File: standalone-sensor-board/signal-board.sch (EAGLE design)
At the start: 32 parts, among them Q1 QRE1113, Q2 QRE1113, Q3 QRE1113, Q4 QRE1113, Q5 QRE1113, Q6 QRE1113, Q7 QRE1113, U1 CD4051BE

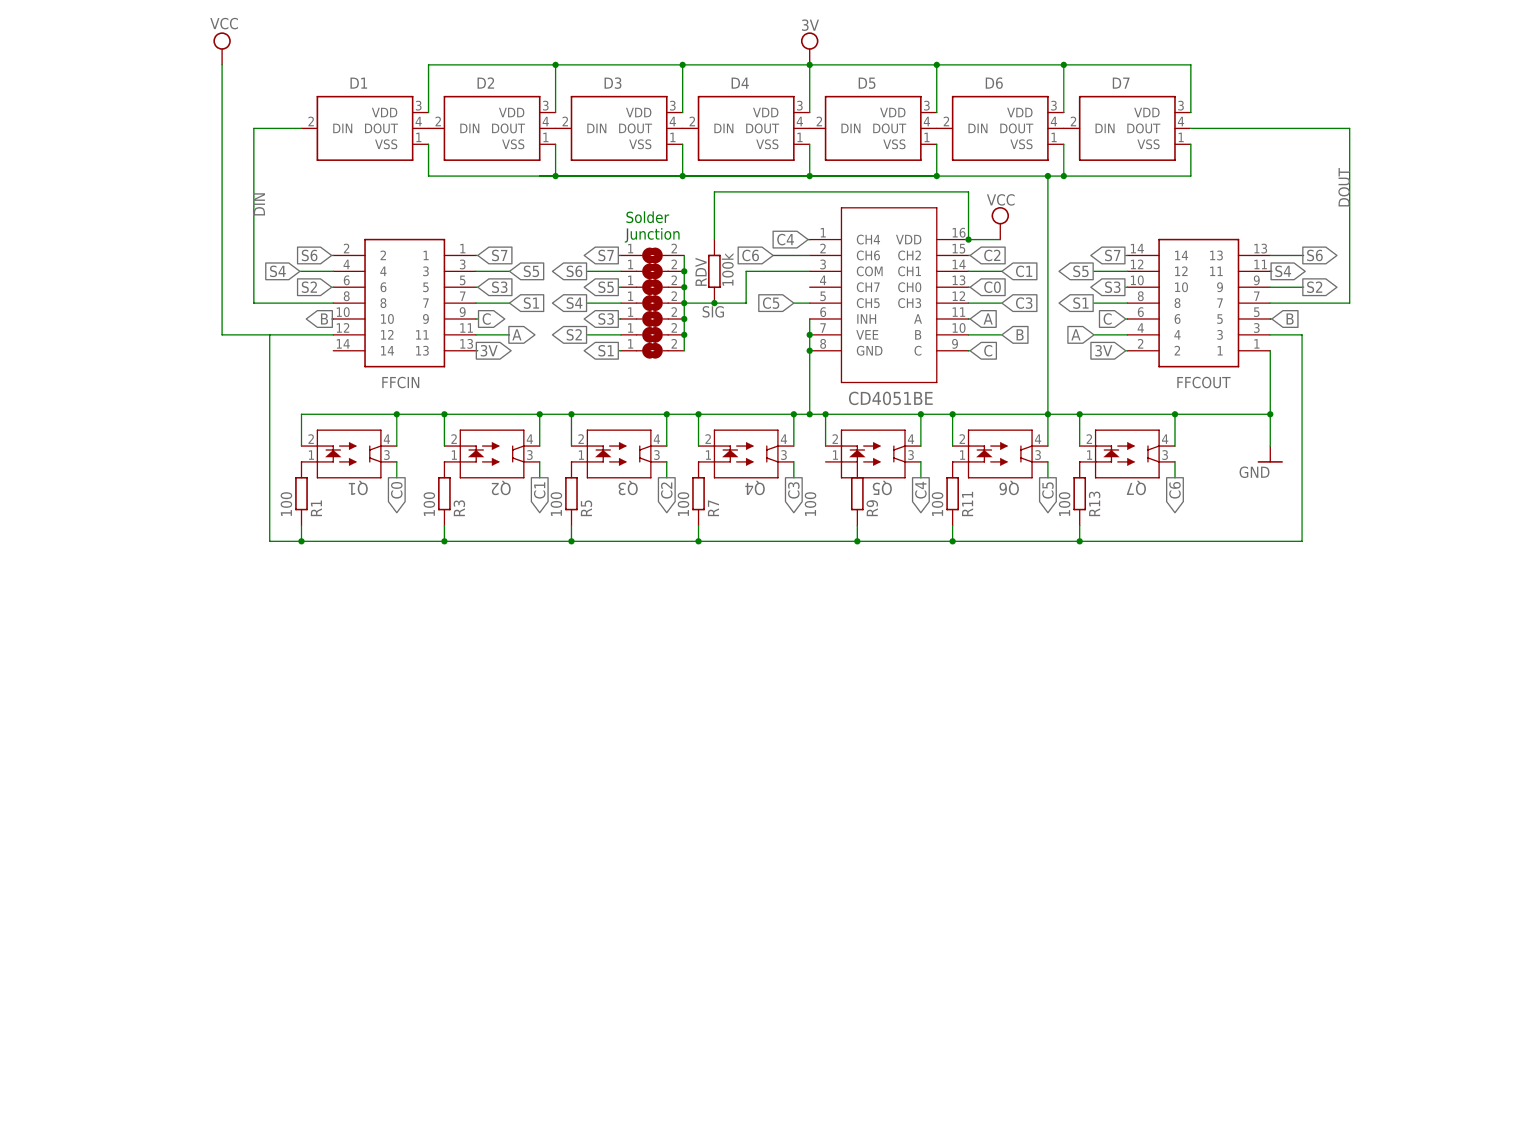
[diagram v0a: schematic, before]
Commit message: rough layout
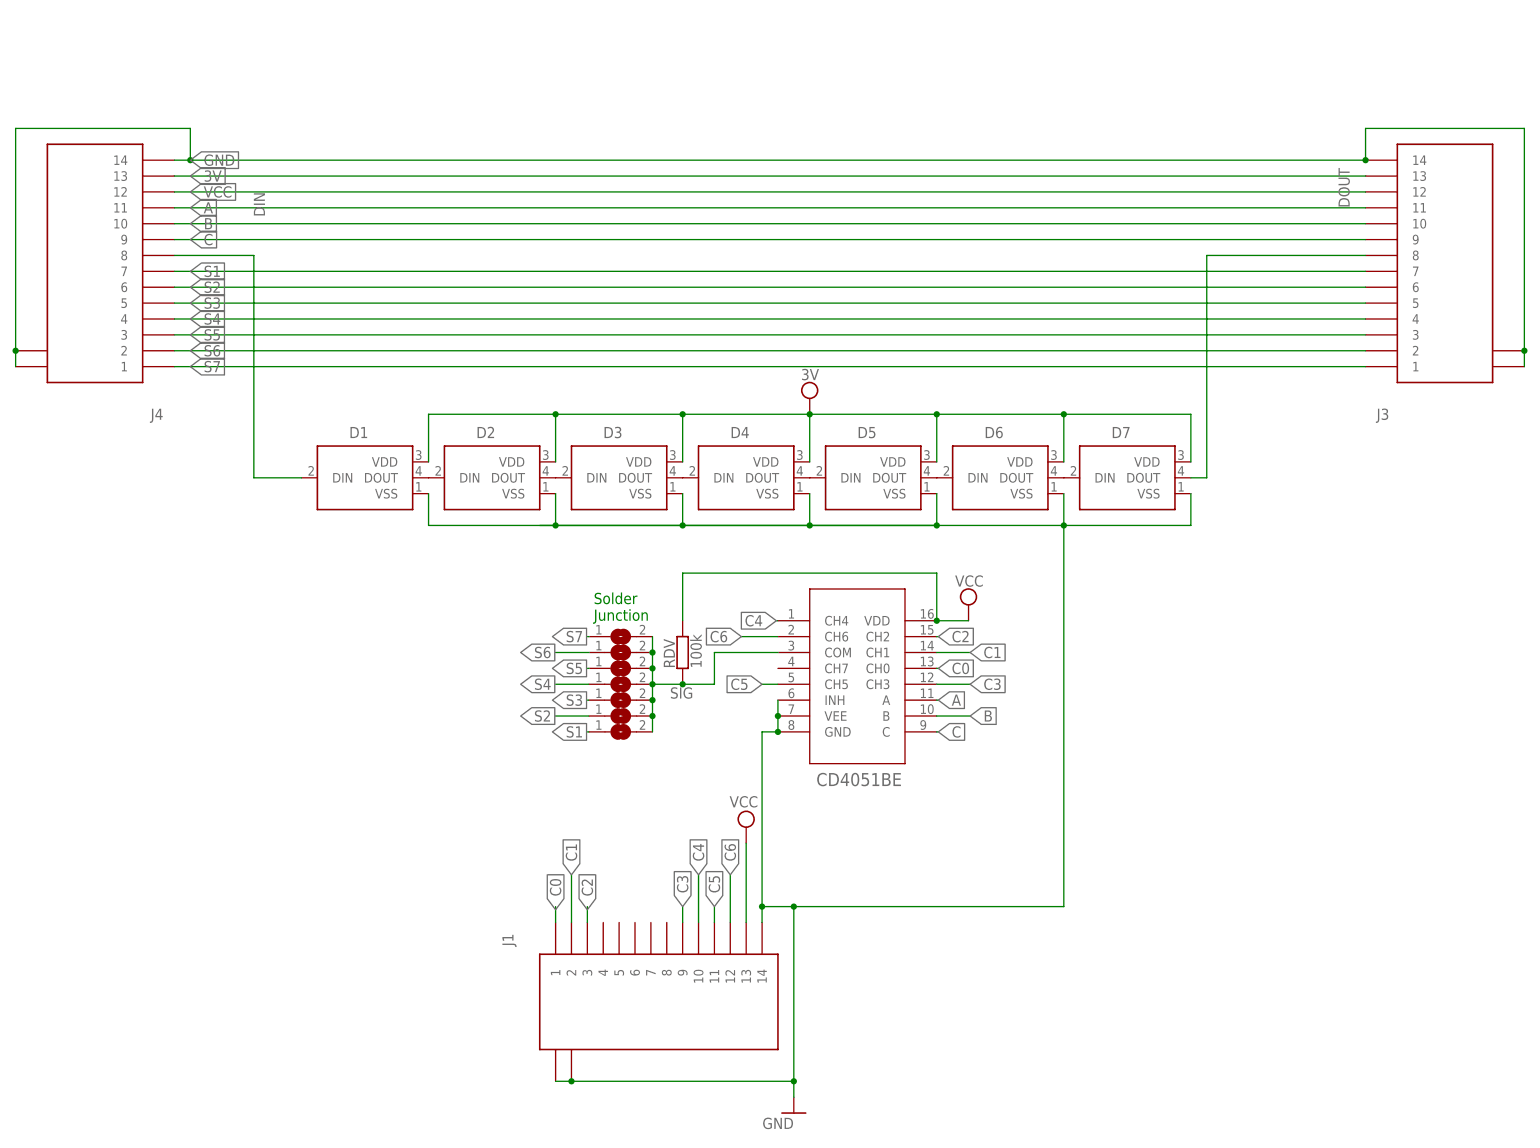
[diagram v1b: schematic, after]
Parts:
- removed FFCIN, FFCOUT: 52806-1410, 52806-1410:52806-1410
- removed Q1, Q2, Q3, Q4, Q5, Q6, Q7: QRE1113, qre1113:QRE1113
- removed R1, R11, R13, R3, R5, R7, R9: 100, rcl:R-EU_0207/10
- added J1, J3, J4: (no value), 686114148922:686114148922
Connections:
- removed net N$1: Q1.1, R1.2
- removed net N$11: Q6.1, R11.2
- removed net N$13: Q7.1, R13.2
- removed net N$2: FFCOUT.3, R1.1, R11.1, R13.1, R3.1, R5.1, R7.1, R9.1
- removed net N$3: Q2.1, R3.2
- removed net N$5: Q3.1, R5.2
- removed net N$7: Q4.1, R7.2
- net 3V: now also J3.13, J4.13; no longer FFCIN.13, FFCOUT.2
- net A: now also J3.11, J4.11; no longer FFCIN.11, FFCOUT.4
- net B: now also J3.10, J4.10; no longer FFCIN.10, FFCOUT.5
- net C: now also J3.9, J4.9; no longer FFCIN.9, FFCOUT.6
- net C0: now also J1.1; no longer Q1.3
- net C1: now also J1.2; no longer Q2.3
- net C2: now also J1.3; no longer Q3.3
- net C3: now also J1.9; no longer Q4.3
- net C4: now also J1.10; no longer Q5.3
- net C5: now also J1.11; no longer Q6.3
- net C6: now also J1.12; no longer Q7.3
- net DIN: now also J4.8; no longer FFCIN.8
- net DOUT: now also J3.8; no longer FFCOUT.7
- net GND: now also J1.14, J1.MP1, J1.MP2, J3.14, J3.MP1, J3.MP2, J4.14, J4.MP1, J4.MP2; no longer FFCOUT.1, Q1.2, Q1.4, Q2.2, Q2.4, Q3.2, Q3.4, Q4.2, Q4.4, Q5.2, Q5.4, Q6.2, Q6.4, Q7.2, Q7.4
- net S1: now also J3.7, J4.7; no longer FFCIN.7, FFCOUT.8
- net S2: now also J3.6, J4.6; no longer FFCIN.6, FFCOUT.9
- net S3: now also J3.5, J4.5; no longer FFCIN.5, FFCOUT.10
- net S4: now also J3.4, J4.4; no longer FFCIN.4, FFCOUT.11
- net S5: now also J3.3, J4.3; no longer FFCIN.3, FFCOUT.12
- net S6: now also J3.2, J4.2; no longer FFCIN.2, FFCOUT.13
- net S7: now also J3.1, J4.1; no longer FFCIN.1, FFCOUT.14
- net VCC: now also J1.13, J3.12, J4.12; no longer FFCIN.12
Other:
- moved on the sheet: D1, D2, D3, D4, D5, D6, D7, RDV
